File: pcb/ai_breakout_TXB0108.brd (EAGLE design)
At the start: 15.2 x 25.4 mm, 8 parts, among them J1 1X10, J2 1X10

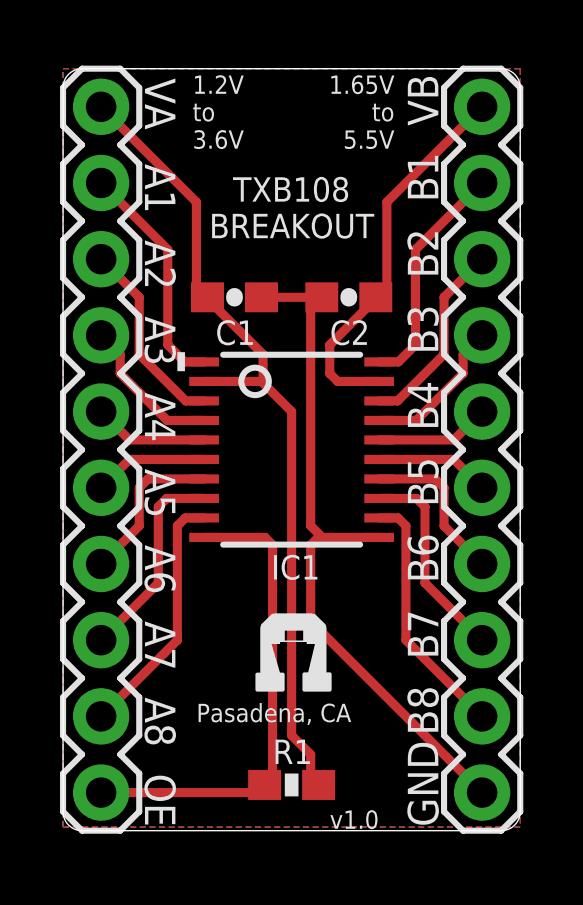
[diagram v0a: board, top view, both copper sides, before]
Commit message: small update schematic
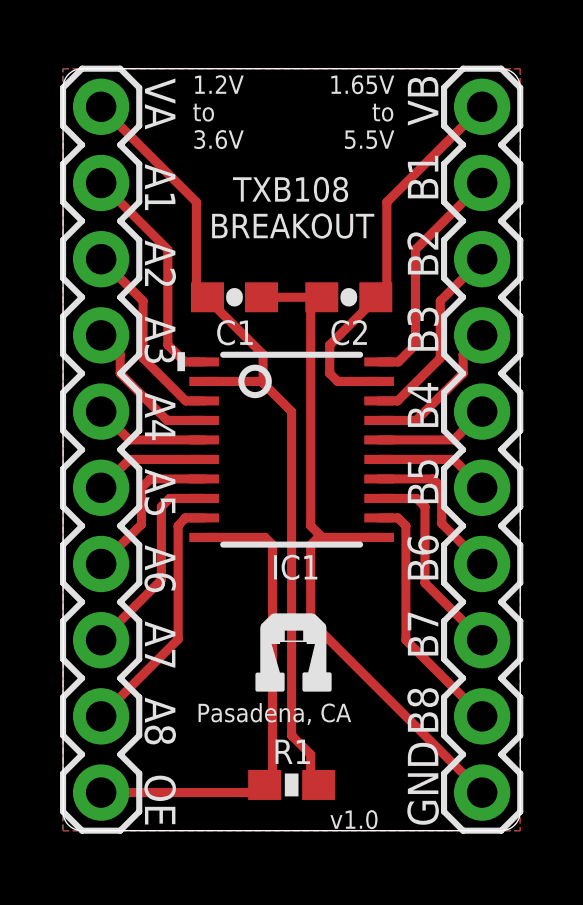
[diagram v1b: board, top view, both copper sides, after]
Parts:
- IC1: value (none) -> TXB0108
- J2: value 1X10 -> 1X10NOFIRST; device Ai_Connectors:1X10 -> Ai_Connectors:1X10-NOFIRST
- moved J1 12.7 mm to (14.0, 12.7)
- moved J2 12.7 mm to (1.27, 12.7)
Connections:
- net A1: now also J2.2; no longer J1.9
- net A2: now also J2.3; no longer J1.8
- net A3: now also J2.4; no longer J1.7
- net A4: now also J2.5; no longer J1.6
- net A5: now also J2.6; no longer J1.5
- net A6: now also J2.7; no longer J1.4
- net A7: now also J2.8; no longer J1.3
- net A8: now also J2.9; no longer J1.2
- net B1: now also J1.9; no longer J2.2
- net B2: now also J1.8; no longer J2.3
- net B3: now also J1.7; no longer J2.4
- net B4: now also J1.6; no longer J2.5
- net B5: now also J1.5; no longer J2.6
- net B6: now also J1.4; no longer J2.7
- net B7: now also J1.3; no longer J2.8
- net B8: now also J1.2; no longer J2.9
- net GND: now also J1.1; no longer J2.10
- net OE: now also J2.10; no longer J1.1
- net VCC-A: now also J2.1; no longer J1.10
- net VCC-B: now also J1.10; no longer J2.1
